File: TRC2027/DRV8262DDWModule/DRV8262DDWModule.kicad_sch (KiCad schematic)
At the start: 9 parts, among them J1 XT30, J2 XT30, J3 Conn_01x05_Pin, U1 DRV8262DDWR

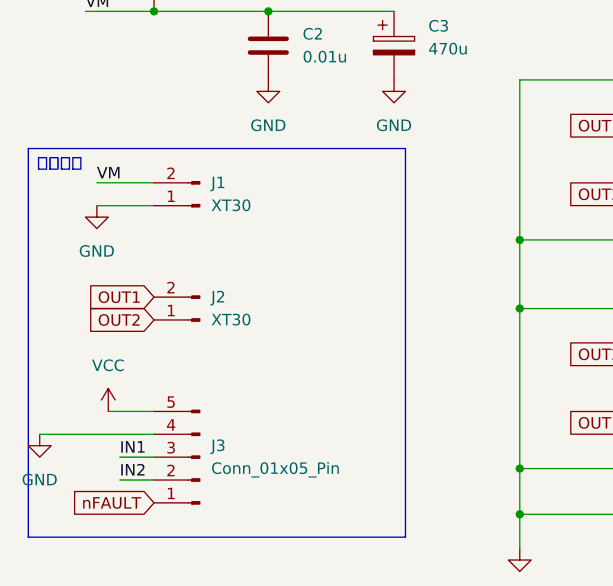
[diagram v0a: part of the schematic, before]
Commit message: add
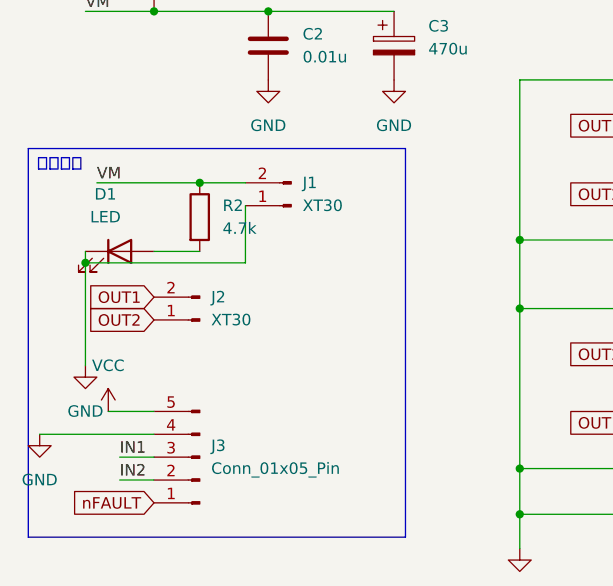
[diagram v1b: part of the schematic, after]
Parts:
- added D1: LED, LED_THT:LED_D5.0mm, symbol Device:LED
- added R2: 4.7k, Resistor_THT:R_Axial_DIN0207_L6.3mm_D2.5mm_P10.16mm_Horizontal, symbol Device:R
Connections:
- net GND: now also D1.1 (K)
- net VM: now also R2.1
- new net: D1.2 (A), R2.2
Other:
- moved on the sheet: J1
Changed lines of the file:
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@@
+	)
+	(junction
+		(at 60.96 87.63)
+		(diameter 0)
+		(color 0 0 0 0)
 	)
 	(junction
@@
 	)
 	(junction
+		(at 48.26 96.52)
+		(diameter 0)
+		(color 0 0 0 0)
+	)
+	(junction
 		(at 111.76 88.9)
 		(diameter 0)
@@
 	(wire
 		(pts
+			(xy 48.26 96.52) (xy 66.04 96.52)
+		)
+		(stroke
+			(width 0)
+			(type default)
+		)
+	)
+	(wire
+		(pts
 			(xy 119.38 83.82) (xy 111.76 83.82)
 		)
@@
 	(wire
 		(pts
-			(xy 49.53 87.63) (xy 55.88 87.63)
+			(xy 49.53 87.63) (xy 60.96 87.63)
 		)
 		(stroke
@@
 	(wire
 		(pts
+			(xy 48.26 95.25) (xy 48.26 96.52)
+		)
+		(stroke
+			(width 0)
+			(type default)
+		)
+	)
+	(wire
+		(pts
 			(xy 111.76 109.22) (xy 119.38 109.22)
 		)
@@
 	(wire
 		(pts
+			(xy 60.96 87.63) (xy 66.04 87.63)
+		)
+		(stroke
+			(width 0)
+			(type default)
+		)
+	)
+	(wire
+		(pts
 			(xy 111.76 116.84) (xy 111.76 114.3)
 		)
@@
 	(wire
 		(pts
-			(xy 49.53 90.17) (xy 55.88 90.17)
-		)
-		(stroke
-			(width 0)
-			(type default)
-		)
-	)
-	(wire
-		(pts
 			(xy 114.3 96.52) (xy 119.38 96.52)
 		)
@@
 	(wire
 		(pts
+			(xy 48.26 107.95) (xy 48.26 96.52)
+		)
+		(stroke
+			(width 0)
+			(type default)
+		)
+	)
+	(wire
+		(pts
 			(xy 185.42 114.3) (xy 189.23 114.3)
 		)
@@
 	(wire
 		(pts
+			(xy 55.88 95.25) (xy 60.96 95.25)
+		)
+		(stroke
+			(width 0)
+			(type default)
+		)
+	)
+	(wire
+		(pts
 			(xy 242.57 113.03) (xy 242.57 119.38)
 		)
@@
 		(pts
 			(xy 111.76 104.14) (xy 111.76 106.68)
+		)
+		(stroke
+			(width 0)
+			(type default)
+		)
+	)
+	(wire
+		(pts
+			(xy 66.04 96.52) (xy 66.04 90.17)
 		)
 		(stroke
@@
 	)
 	(symbol
+		(lib_id "Device:LED")
+		(at 52.07 95.25 0)
+		(unit 1)
+		(exclude_from_sim no)
+		(in_bom yes)
+		(on_board yes)
+		(dnp no)
+		(fields_autoplaced yes)
+		(property "Reference" "D1"
+			(at 50.4825 88.9 0)
+			(effects
+				(font
+					(size 1.27 1.27)
+				)
+			)
+		)
+		(property "Value" "LED"
+			(at 50.4825 91.44 0)
+			(effects
+				(font
+					(size 1.27 1.27)
+				)
+			)
+		)
+		(property "Footprint" "LED_THT:LED_D5.0mm"
+			(at 52.07 95.25 0)
+			(effects
+				(font
+					(size 1.27 1.27)
+				)
+				(hide yes)
+			)
+		)
+		(property "Datasheet" "~"
+			(at 52.07 95.25 0)
+			(effects
+				(font
+					(size 1.27 1.27)
+				)
+				(hide yes)
+			)
+		)
+		(property "Description" "Light emitting diode"
+			(at 52.07 95.25 0)
+			(effects
+				(font
+					(size 1.27 1.27)
+				)
+				(hide yes)
+			)
+		)
+		(property "Sim.Pins" "1=K 2=A"
+			(at 52.07 95.25 0)
+			(effects
+				(font
+					(size 1.27 1.27)
+				)
+				(hide yes)
+			)
+		)
+		(pin "1"
+		)
+		(pin "2"
+		)
+		(instances
+			(project ""
+				(path "/276fb546-4d9d-4e3f-a384-4b93d5480cfc"
+					(reference "D1")
+					(unit 1)
+				)
+			)
+		)
+	)
+	(symbol
+		(lib_id "Device:R")
+		(at 60.96 91.44 0)
+		(unit 1)
+		(exclude_from_sim no)
+		(in_bom yes)
+		(on_board yes)
+		(dnp no)
+		(fields_autoplaced yes)
+		(property "Reference" "R2"
+			(at 63.5 90.1699 0)
+			(effects
+				(font
+					(size 1.27 1.27)
+				)
+				(justify left)
+			)
+		)
+		(property "Value" "4.7k"
+			(at 63.5 92.7099 0)
+			(effects
+				(font
+					(size 1.27 1.27)
+				)
+				(justify left)
+			)
+		)
+		(property "Footprint" "Resistor_THT:R_Axial_DIN0207_L6.3mm_D2.5mm_P10.16mm_Horizontal"
+			(at 59.182 91.44 90)
+			(effects
+				(font
+					(size 1.27 1.27)
+				)
+				(hide yes)
+			)
+		)
+		(property "Datasheet" "~"
+			(at 60.96 91.44 0)
+			(effects
+				(font
+					(size 1.27 1.27)
+				)
+				(hide yes)
+			)
+		)
+		(property "Description" "Resistor"
+			(at 60.96 91.44 0)
+			(effects
+				(font
+					(size 1.27 1.27)
+				)
+				(hide yes)
+			)
+		)
+		(pin "2"
+		)
+		(pin "1"
+		)
+		(instances
+			(project ""
+				(path "/276fb546-4d9d-4e3f-a384-4b93d5480cfc"
+					(reference "R2")
+					(unit 1)
+				)
+			)
+		)
+	)
+	(symbol
 		(lib_id "power:GND")
 		(at 217.17 129.54 0)
@@
 	(symbol
 		(lib_id "Connector:Conn_01x02_Pin")
-		(at 60.96 90.17 180)
+		(at 71.12 90.17 180)
 		(unit 1)
 		(exclude_from_sim no)
@@
 		(fields_autoplaced yes)
 		(property "Reference" "J1"
-			(at 62.23 87.6299 0)
+			(at 72.39 87.6299 0)
 			(effects
 				(font
@@
 		)
 		(property "Value" "XT30"
-			(at 62.23 90.1699 0)
+			(at 72.39 90.1699 0)
 			(effects
 				(font
@@
 		)
 		(property "Footprint" "Connector_AMASS:AMASS_XT30PW-F_1x02_P2.50mm_Horizontal"
-			(at 60.96 90.17 0)
+			(at 71.12 90.17 0)
 			(effects
 				(font
@@
 		)
 		(property "Datasheet" "~"
-			(at 60.96 90.17 0)
+			(at 71.12 90.17 0)
 			(effects
 				(font
@@
 		)
 		(property "Description" "Generic connector, single row, 01x02, script generated"
-			(at 60.96 90.17 0)
+			(at 71.12 90.17 0)
 			(effects
 				(font
@@
 	(symbol
 		(lib_id "power:GND")
-		(at 49.53 90.17 0)
+		(at 48.26 107.95 0)
 		(unit 1)
 		(exclude_from_sim no)
@@
 		(fields_autoplaced yes)
 		(property "Reference" "#PWR09"
-			(at 49.53 96.52 0)
+			(at 48.26 114.3 0)
 			(effects
 				(font
@@
 		)
 		(property "Value" "GND"
-			(at 49.53 95.25 0)
+			(at 48.26 113.03 0)
 			(effects
 				(font
@@
 		)
 		(property "Footprint" ""
-			(at 49.53 90.17 0)
+			(at 48.26 107.95 0)
 			(effects
 				(font
@@
 		)
 		(property "Datasheet" ""
-			(at 49.53 90.17 0)
+			(at 48.26 107.95 0)
 			(effects
 				(font
@@
 		)
 		(property "Description" "Power symbol creates a global label with name \"GND\" , ground"
-			(at 49.53 90.17 0)
-			(effects
-				(font
+			(at 48.26 107.95 0)
+			(effects
+				(font
